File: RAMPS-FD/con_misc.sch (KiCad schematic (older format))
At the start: 11 parts, among them K201 SER1, K202 SER2, K203 SER3, K204 SER4, P211 I2C, P213 AUX-4, P214 AUX-2, P215 AUX-3, P216 SERIAL

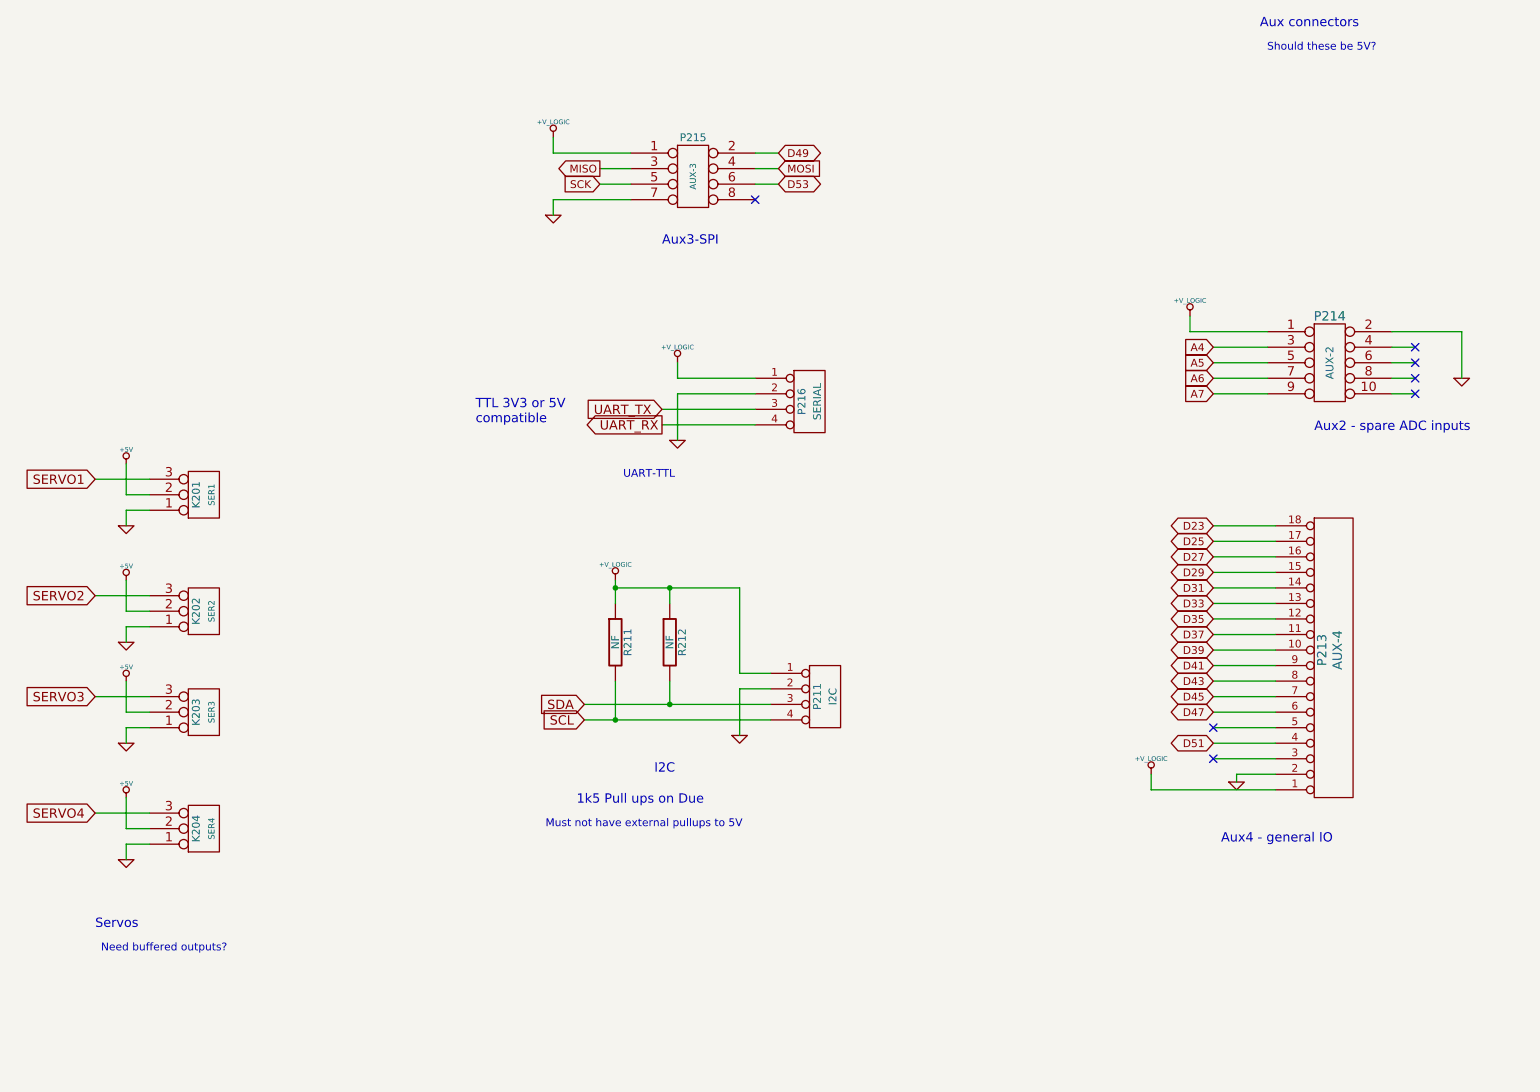
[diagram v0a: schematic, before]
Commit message: RAMPS-FD update
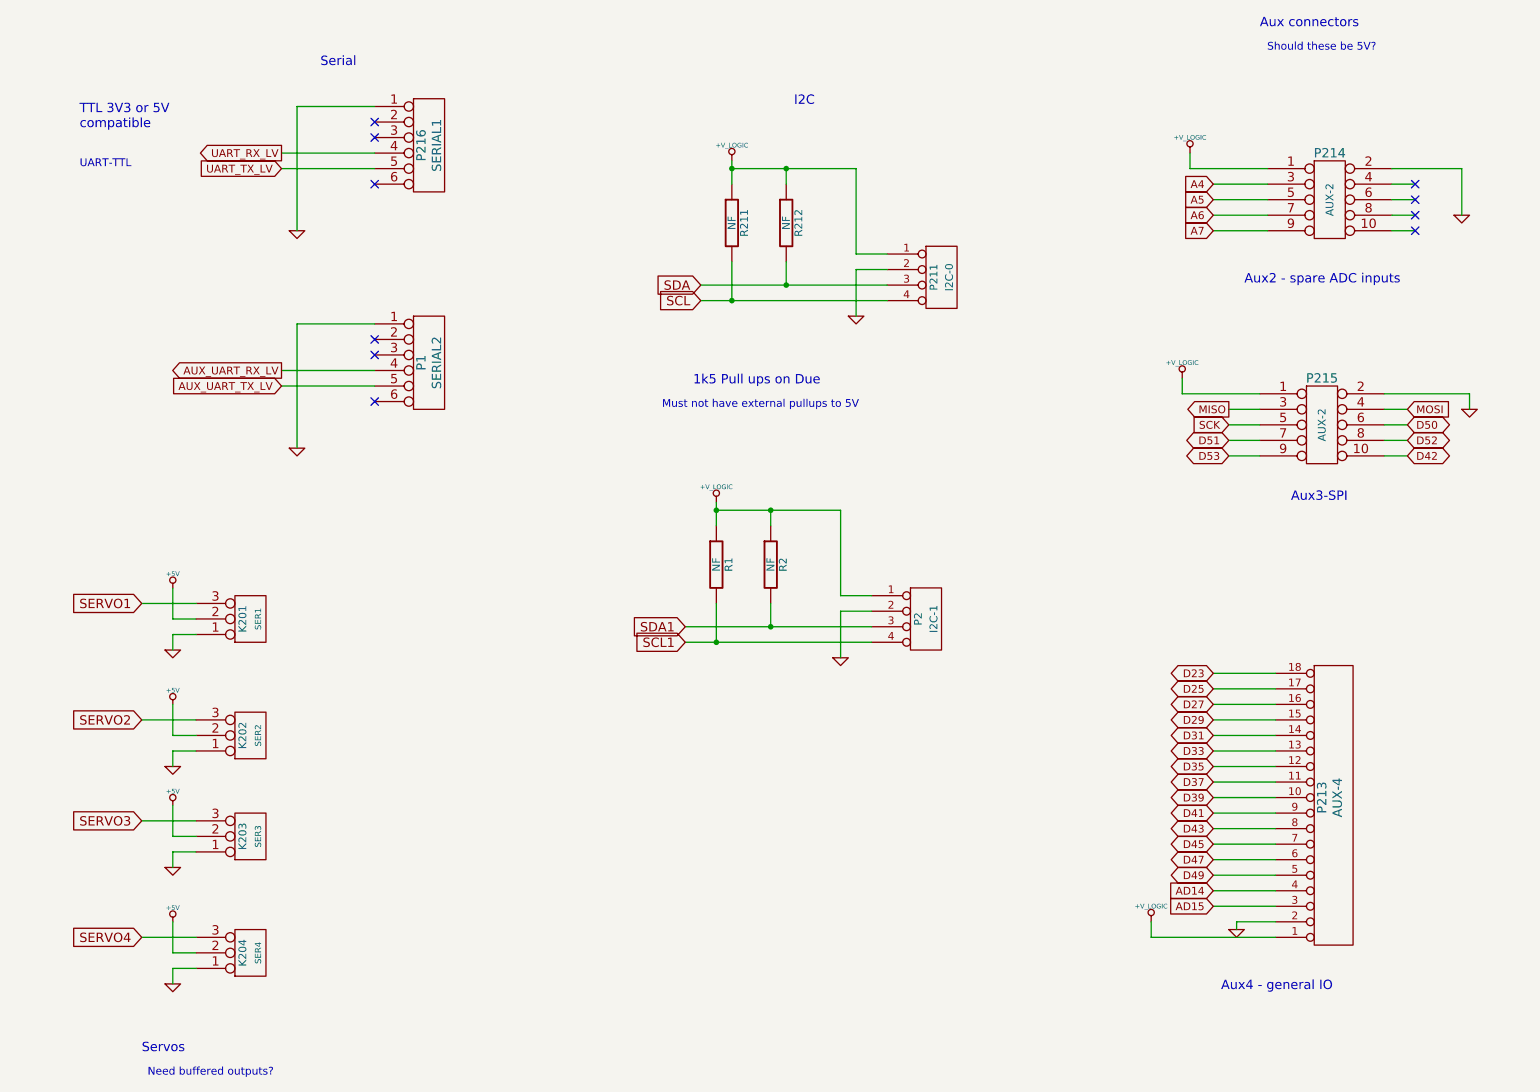
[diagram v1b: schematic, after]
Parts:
- removed P215: AUX-3, symbol CONN_4X2
- removed P216: SERIAL, symbol CONN_4
- added P1: SERIAL2, symbol CONN_6
- added P2: I2C-1, symbol CONN_4
- added P215: AUX-2, symbol CONN_5X2
- added P216: SERIAL1, symbol CONN_6
- added R1, R2: NF, symbol R
- P211: value I2C -> I2C-0
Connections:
- net +V_LOGIC: now also P2.1 (P1), P215.1, R1.1, R2.1
- net D49: now also P213.5 (P5)
- net D51: now also P215.7; no longer P213.4 (P4)
- net D53: now also P215.9
- net GND: now also P1.1, P2.2 (P2), P215.2, P216.1
- net MISO: now also P215.3
- net MOSI: now also P215.4
- net SCK: now also P215.5
- net AD15: now reaches P213.3 (P3)
- new net AD14: P213.4 (P4)
- new net AUX_UART_RX_LV: P1.4
- new net AUX_UART_TX_LV: P1.5
- new net D42: P215.10
- new net D50: P215.6
- new net D52: P215.8
- new net SCL1: P2.4 (P4), R1.2
- new net SDA1: P2.3 (P3), R2.2
- new net UART_RX_LV: P216.4
- new net UART_TX_LV: P216.5
- no-connect marks 7 -> 10
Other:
- note added: "Serial"
- moved on the sheet: K201, K202, K203, K204, P211, P213, P214, R211, R212

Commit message: Updates to RAMPS-FD
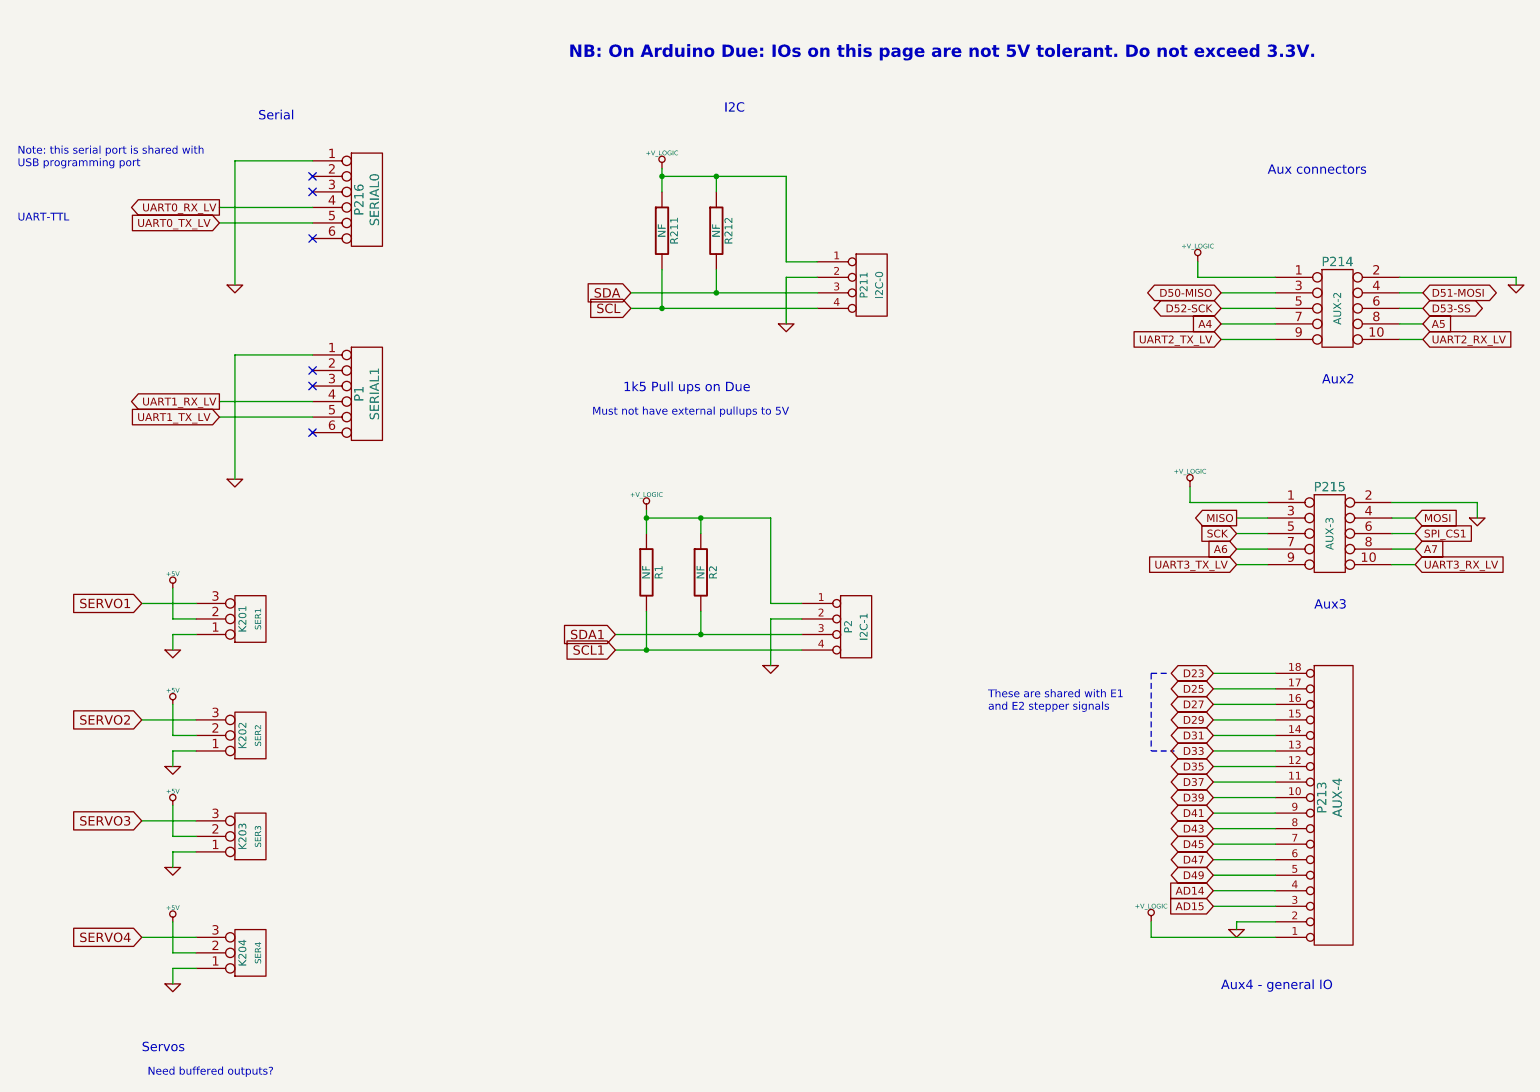
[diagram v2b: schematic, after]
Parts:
- P1: value SERIAL2 -> SERIAL1
- P215: value AUX-2 -> AUX-3
- P216: value SERIAL1 -> SERIAL0
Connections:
- net D51 is gone; now on net A6: P215.7
- net D52 is gone; now on net A7: P215.8
- net A4: now also P214.7; no longer P214.3
- net A5: now also P214.8; no longer P214.5
- net A6: no longer P214.7
- net A7: no longer P214.9
- net UART2_RX_LV: now reaches P214.10
- net D51-MOSI: now reaches P214.4
- net D53-SS: now reaches P214.6
- net AUX_UART_RX_LV renamed UART1_RX_LV
- net AUX_UART_TX_LV renamed UART1_TX_LV
- net D42 renamed UART3_RX_LV
- net D50 renamed SPI_CS1
- net D53 renamed UART3_TX_LV
- net UART_RX_LV renamed UART0_RX_LV
- net UART_TX_LV renamed UART0_TX_LV
- new net D50-MISO: P214.3
- new net D52-SCK: P214.5
- new net UART2_TX_LV: P214.9
- no-connect marks 10 -> 6
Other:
- note added: "Aux2"
- note added: "Aux3"
- note added: "NB: On Arduino Due: IOs on this page are not 5V tolerant. Do not exceed 3.3V."
- note added: "Note: this serial port is shared with\nUSB programming port"
- note added: "These are shared with E1 \nand E2 stepper signals"
- note removed: "Aux2 - spare ADC inputs"
- note removed: "Aux3-SPI"
- note removed: "Should these be 5V?"
- note removed: "TTL 3V3 or 5V\ncompatible"
- moved on the sheet: P1, P2, P211, P214, P215, P216, R1, R2, R211, R212
